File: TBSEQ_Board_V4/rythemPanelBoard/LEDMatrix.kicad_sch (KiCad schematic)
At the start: 32 parts

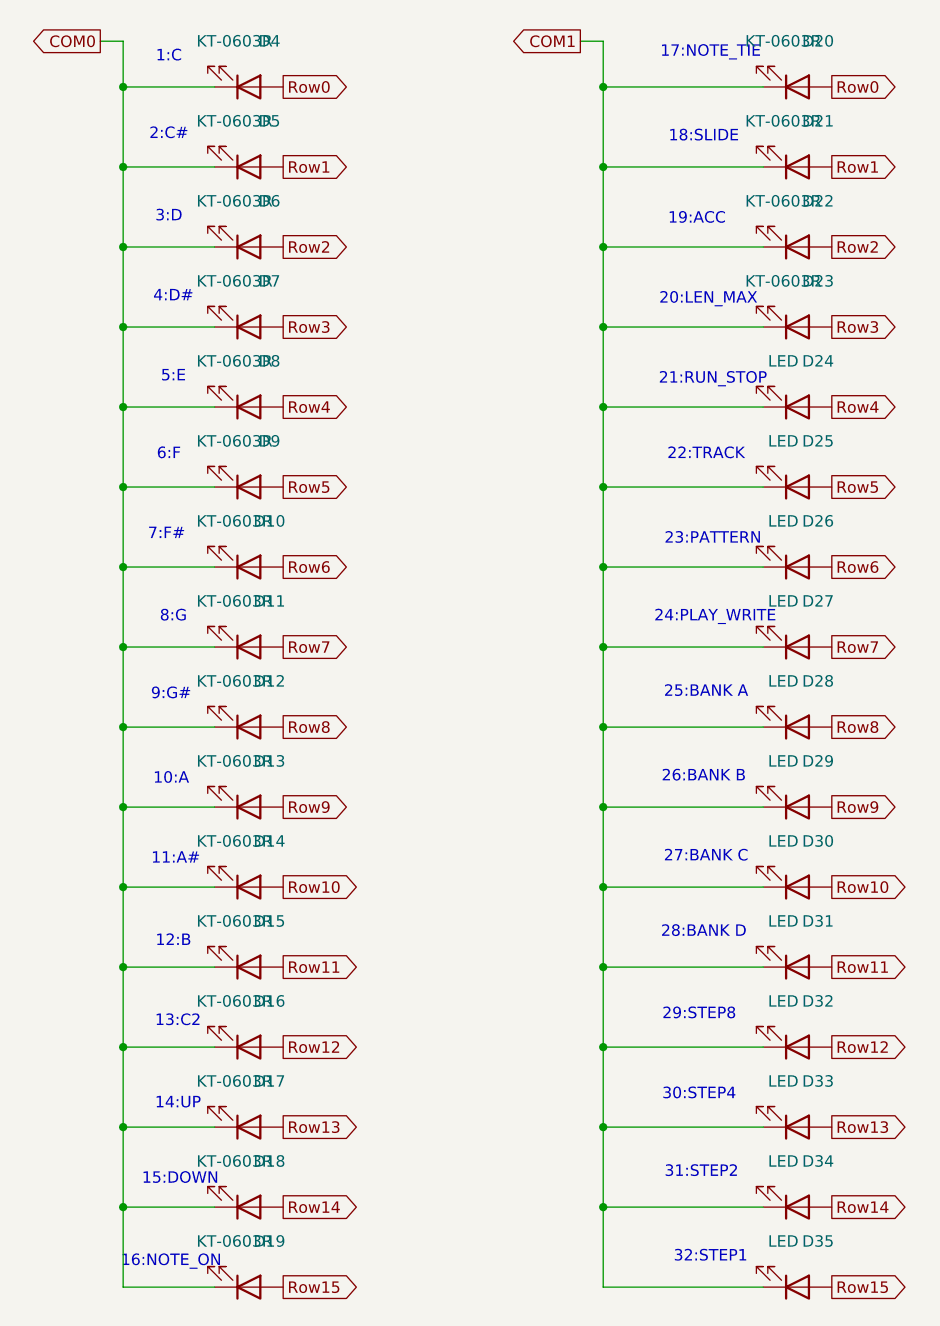
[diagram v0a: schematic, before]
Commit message: TBSEQ_BoardV4
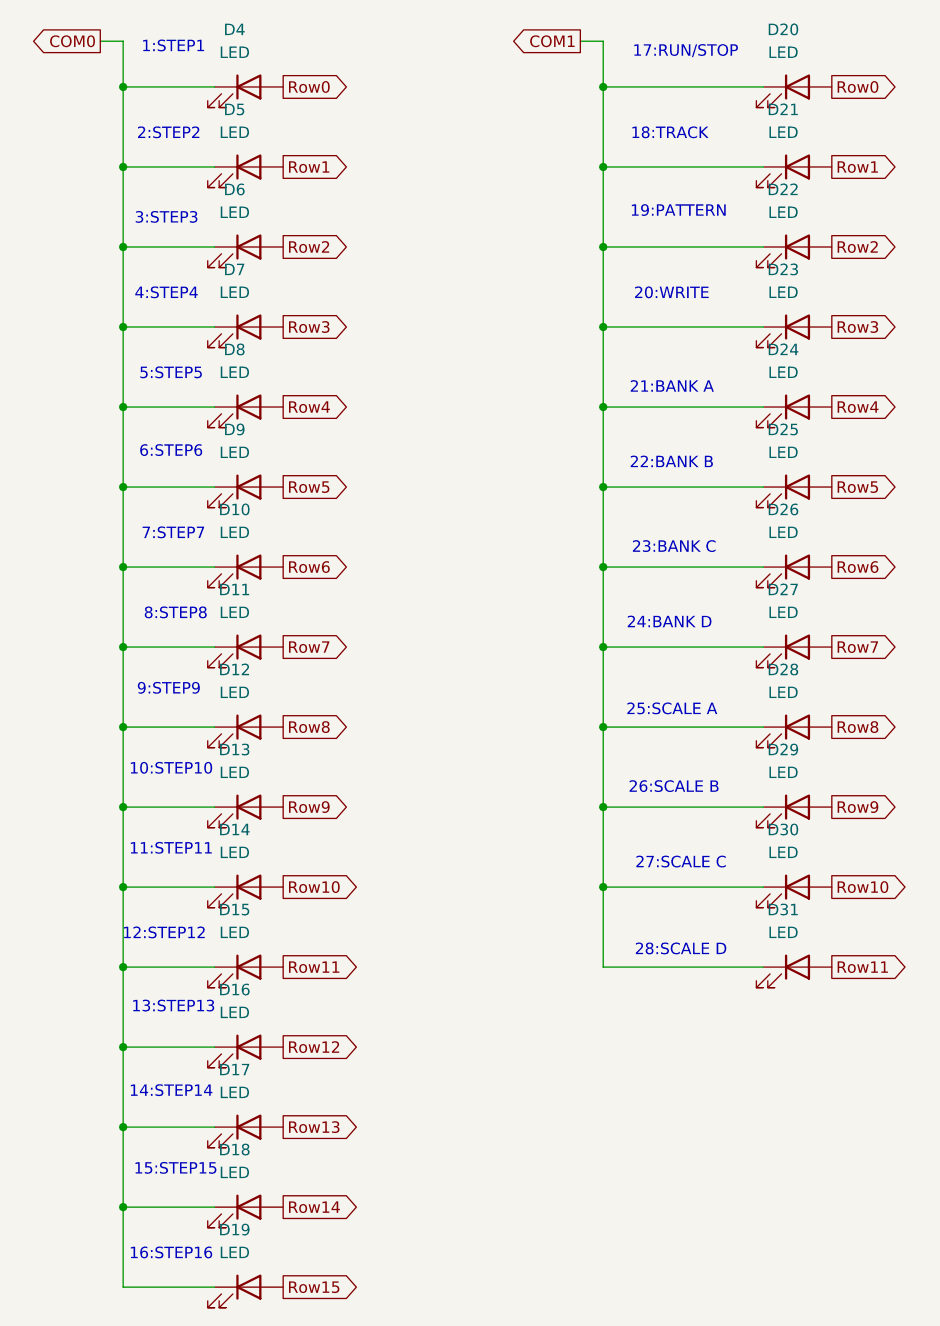
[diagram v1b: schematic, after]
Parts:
- removed D32, D33, D34, D35: LED, LED_SMD:LED_0603_1608Metric_Pad1.05x0.95mm_HandSolder, symbol Device:LED
- D10, D11, D12, D13, D14, D15, D16, D17, D18, D19, D20, D21, D22, D23, D4, D5, D6, D7, D8, D9: value KT-0603R -> LED
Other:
- note added: "10:STEP10"
- note added: "11:STEP11"
- note added: "12:STEP12"
- note added: "13:STEP13"
- note added: "14:STEP14"
- note added: "15:STEP15"
- note added: "16:STEP16"
- note added: "17:RUN/STOP"
- note added: "18:TRACK"
- note added: "19:PATTERN"
- note added: "1:STEP1"
- note added: "20:WRITE"
- note added: "21:BANK A"
- note added: "22:BANK B"
- note added: "23:BANK C"
- note added: "24:BANK D"
- note added: "25:SCALE A"
- note added: "26:SCALE B"
- note added: "27:SCALE C"
- note added: "28:SCALE D"
- note added: "2:STEP2"
- note added: "3:STEP3"
- note added: "4:STEP4"
- note added: "5:STEP5"
- note added: "6:STEP6"
- note added: "7:STEP7"
- note added: "8:STEP8"
- note added: "9:STEP9"
- note removed: "10:A"
- note removed: "11:A#"
- note removed: "12:B"
- note removed: "13:C2"
- note removed: "14:UP"
- note removed: "15:DOWN"
- note removed: "16:NOTE_ON"
- note removed: "17:NOTE_TIE"
- note removed: "18:SLIDE"
- note removed: "19:ACC"
- note removed: "1:C"
- note removed: "20:LEN_MAX"
- note removed: "21:RUN_STOP"
- note removed: "22:TRACK"
- note removed: "23:PATTERN"
- note removed: "24:PLAY_WRITE"
- note removed: "25:BANK A"
- note removed: "26:BANK B"
- note removed: "27:BANK C"
- note removed: "28:BANK D"
- note removed: "29:STEP8"
- note removed: "2:C#"
- note removed: "30:STEP4"
- note removed: "31:STEP2"
- note removed: "32:STEP1"
- note removed: "3:D"
- note removed: "4:D#"
- note removed: "5:E"
- note removed: "6:F"
- note removed: "7:F#"
- note removed: "8:G"
- note removed: "9:G#"
